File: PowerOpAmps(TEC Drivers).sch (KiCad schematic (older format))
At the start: 23 parts, among them U301 OPA569AIDWPR, U302 OPA569AIDWPR

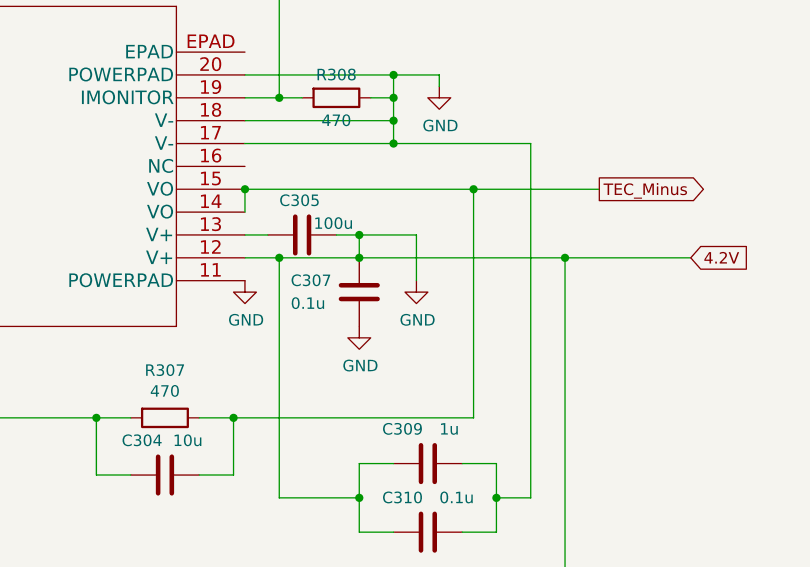
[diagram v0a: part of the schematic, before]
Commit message: SOLVED: GND and 4.2V
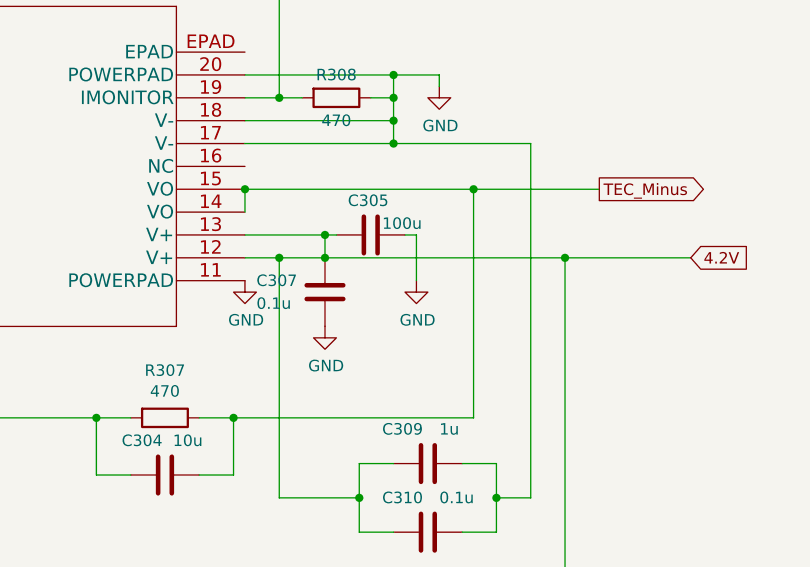
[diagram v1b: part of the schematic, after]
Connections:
- net GND: now also C305.2, U301.13 (V+)
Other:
- moved on the sheet: C307
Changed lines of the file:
@@
 	7500 2500 7500 2400
 Wire Wire Line
-	7500 2600 7600 2600
-Wire Wire Line
-	8000 2600 8000 2700
-Wire Wire Line
-	8000 2600 8250 2600
-Connection ~ 8000 2600
+	7850 2600 7850 2700
 $Comp
 L power:GND #PWR0310
 U 1 1 60C9E215
-P 8000 3000
-F 0 "#PWR0310" H 8000 2750 50  0001 C CNN
-F 1 "GND" H 8005 2827 50  0000 C CNN
-F 2 "" H 8000 3000 50  0001 C CNN
-F 3 "" H 8000 3000 50  0001 C CNN
-	1    8000 3000
+P 7850 3000
+F 0 "#PWR0310" H 7850 2750 50  0001 C CNN
+F 1 "GND" H 7855 2827 50  0000 C CNN
+F 2 "" H 7850 3000 50  0001 C CNN
+F 3 "" H 7850 3000 50  0001 C CNN
+	1    7850 3000
 	1    0    0    -1
 $EndComp
@@
 L Device:C C307
 U 1 1 60C9E72B
-P 8000 2850
-F 0 "C307" H 7700 2900 50  0000 L CNN
-F 1 "0.1u" H 7700 2800 50  0000 L CNN
-F 2 "Capacitor_SMD:C_0402_1005Metric" H 8038 2700 50  0001 C CNN
-F 3 "~" H 8000 2850 50  0001 C CNN
-	1    8000 2850
-	1    0    0    -1
-$EndComp
-Connection ~ 8000 2700
+P 7850 2850
+F 0 "C307" H 7550 2900 50  0000 L CNN
+F 1 "0.1u" H 7550 2800 50  0000 L CNN
+F 2 "Capacitor_SMD:C_0402_1005Metric" H 7888 2700 50  0001 C CNN
+F 3 "~" H 7850 2850 50  0001 C CNN
+	1    7850 2850
+	1    0    0    -1
+$EndComp
+Connection ~ 7850 2700
 $Comp
 L power:GND #PWR0308
@@
 	1    0    0    -1
 $EndComp
-$Comp
-L Device:C C305
-U 1 1 60CA0405
-P 7750 2600
-F 0 "C305" V 7600 2500 50  0000 L CNN
-F 1 "100u" V 7700 2650 50  0000 L CNN
-F 2 "Capacitor_SMD:C_0402_1005Metric" H 7788 2450 50  0001 C CNN
-F 3 "~" H 7750 2600 50  0001 C CNN
-	1    7750 2600
-	0    1    1    0
-$EndComp
-Wire Wire Line
-	7900 2600 8000 2600
 Wire Wire Line
 	8250 2600 8250 2800
@@
 	8900 2700 9450 2700
 Wire Wire Line
-	8000 2700 8900 2700
+	7850 2700 8900 2700
 Connection ~ 8900 2700
 Wire Wire Line
@@
 Connection ~ 7650 2700
 Wire Wire Line
-	7650 2700 8000 2700
+	7650 2700 7850 2700
 Wire Wire Line
 	8750 2200 8150 2200
@@
 Text GLabel 7650 1100 2    50   Output ~ 0
 To_Arduino_AtoD_Neg
+$Comp
+L Device:C C305
+U 1 1 60CEBDD3
+P 8050 2600
+F 0 "C305" V 7900 2500 50  0000 L CNN
+F 1 "100u" V 8000 2650 50  0000 L CNN
+F 2 "Capacitor_SMD:C_0402_1005Metric" H 8088 2450 50  0001 C CNN
+F 3 "~" H 8050 2600 50  0001 C CNN
+	1    8050 2600
+	0    1    1    0
+$EndComp
+Wire Wire Line
+	7500 2600 7850 2600
+Wire Wire Line
+	7900 2600 7850 2600
+Connection ~ 7850 2600
+Wire Wire Line
+	8250 2600 8200 2600
 $EndSCHEMATC
